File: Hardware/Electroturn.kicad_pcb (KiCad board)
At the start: 2 copper layers, 122 x 83.1 mm, 45 parts, among them Q1 2N2222, U2 RT9193-3.3, U3 74HC4050D

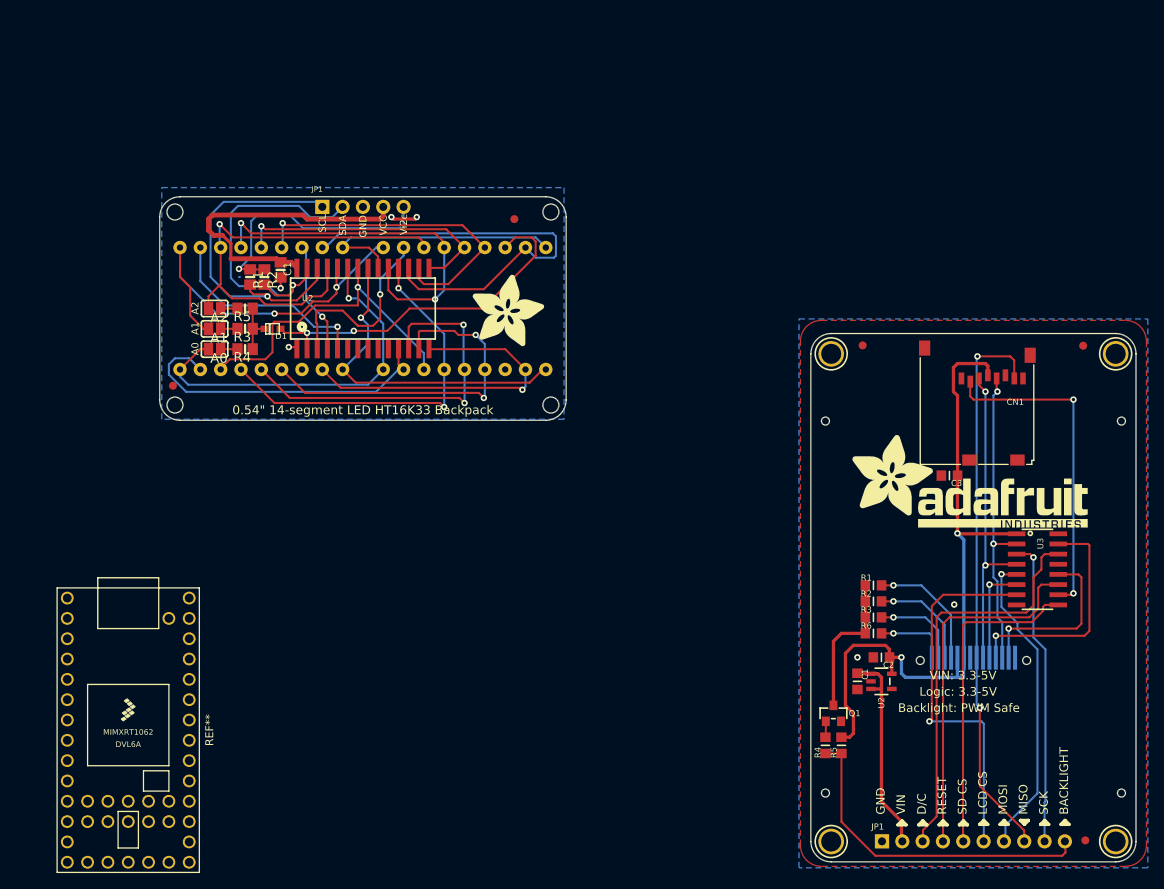
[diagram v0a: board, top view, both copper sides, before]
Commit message: Something like a pcb?
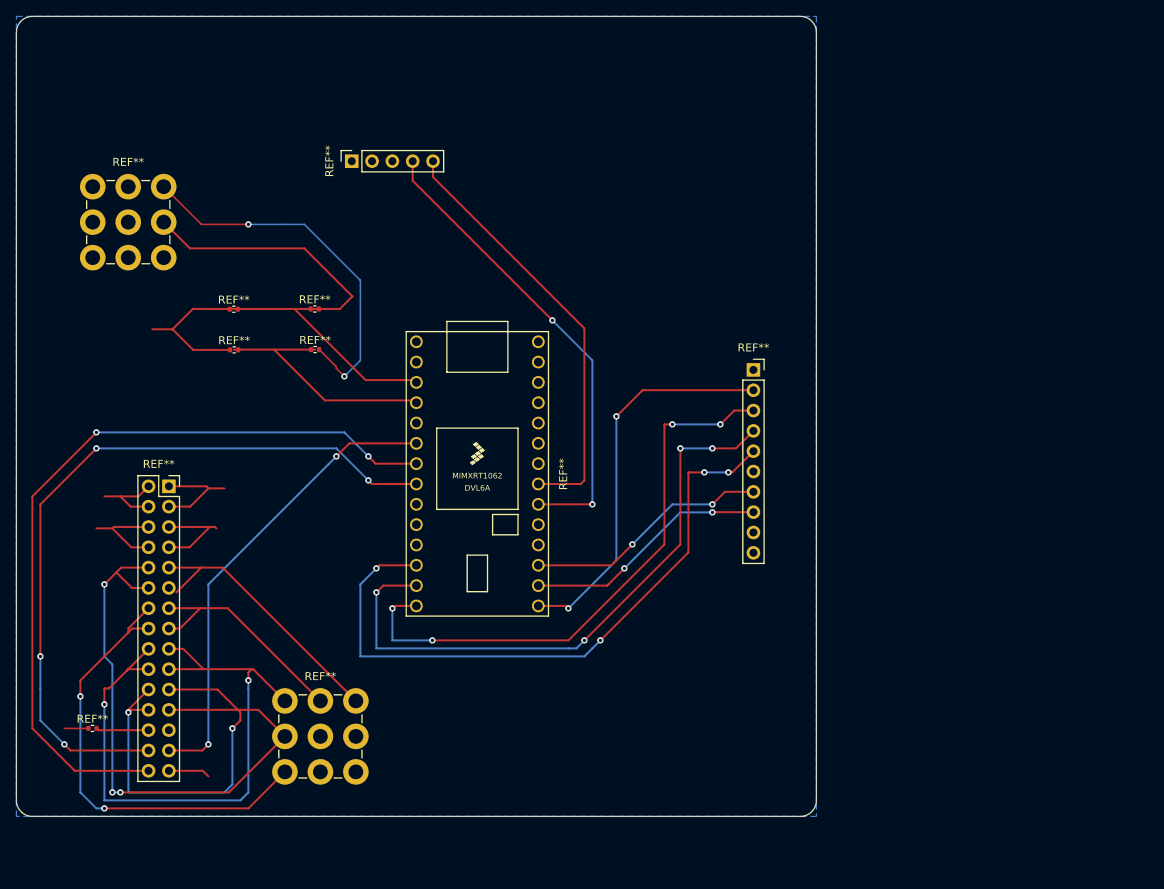
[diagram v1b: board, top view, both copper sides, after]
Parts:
- removed @HOLE0, @HOLE1, @HOLE2, @HOLE3: , 
- removed A0, A1, A2: , Adafruit 0.54 Alphanumeric v0.1:SOLDERJUMPER_REFLOW_NOPASTE
- removed C1: 10uF, Adafruit 0.54 Alphanumeric v0.1:0805-NO
- removed C1, C2, C3: 10uF, Adafruit_2.2_SPI_240x320:_0805MP
- removed CN1: , Adafruit_2.2_SPI_240x320:MICROSD
- removed D1: 1N4148, Adafruit 0.54 Alphanumeric v0.1:SOD-323F
- removed FID1, FID2, FID3: FIDUCIAL"", Adafruit_2.2_SPI_240x320:FIDUCIAL_1MM
- removed JP1: , Adafruit 0.54 Alphanumeric v0.1:1X05_ROUND_70
- removed JP1: , Adafruit_2.2_SPI_240x320:1X10_ROUND70
- removed LED1, LED2: , Adafruit 0.54 Alphanumeric v0.1:SEGMENT_STARTBUST_DUAL_KWA-541CBB
- removed Q1: 2N2222, Adafruit_2.2_SPI_240x320:SOT23-WIDE
- removed R1, R2: 10K, Adafruit 0.54 Alphanumeric v0.1:0805-NO
- removed R1, R2, R3, R6: 10, Adafruit_2.2_SPI_240x320:_0805MP
- removed R3, R4, R5: 47K, Adafruit 0.54 Alphanumeric v0.1:0805-NO
- removed R4: 1K, Adafruit_2.2_SPI_240x320:_0805MP
- removed R5: 10K, Adafruit_2.2_SPI_240x320:_0805MP
- removed U$1, U$2: FIDUCIAL, Adafruit 0.54 Alphanumeric v0.1:FIDUCIAL_1MM
- removed U$2, U$3, U$4, U$5: MOUNTINGHOLE2.5, Adafruit_2.2_SPI_240x320:MOUNTINGHOLE_2.5_PLATED
- removed U$20: , Adafruit_2.2_SPI_240x320:ADAFRUIT_TEXT_30MM
- removed U$3: , Adafruit 0.54 Alphanumeric v0.1:ADAFRUIT_9MM
- removed U1: , Adafruit_2.2_SPI_240x320:TM022HDH26_2.2IN_LCD
- removed U2: , Adafruit 0.54 Alphanumeric v0.1:SOP28_300MIL
- removed U2: RT9193-3.3, Adafruit_2.2_SPI_240x320:SOT23-5
- removed U3: 74HC4050D, Adafruit_2.2_SPI_240x320:SOIC16
- added REF**: Gecko G250x, Connector_PinSocket_2.54mm:PinSocket_2x15_P2.54mm_Vertical, F.Cu at (99.1, 78.7)
- added REF**: Alphanumeric, Connector_PinSocket_2.54mm:PinSocket_1x05_P2.54mm_Vertical, F.Cu at (121.9, 38.1)
- added REF**: Screw Terminal, TerminalBlock_Wuerth:Wuerth_REDCUBE-THR_WP-THRBU_74650194_THR, F.Cu at (118.0, 110.0)
- added REF**: 5k, Resistor_SMD:R_0402_1005Metric, F.Cu at (117.3, 56.6)
- added REF**: Screw Terminal, TerminalBlock_Wuerth:Wuerth_REDCUBE-THR_WP-THRBU_74650194_THR, F.Cu at (94.0, 45.7)
- added REF**: 10k, Resistor_SMD:R_0402_1005Metric, F.Cu at (107.2, 61.7)
- added REF**: 5k, Resistor_SMD:R_0402_1005Metric, F.Cu at (117.3, 61.6)
- added REF**: TFT Display, Connector_PinSocket_2.54mm:PinSocket_1x10_P2.54mm_Vertical, F.Cu at (172.1, 64.2)
- added REF**: 10k, Resistor_SMD:R_0402_1005Metric, F.Cu at (107.2, 56.6)
- added REF**: 2.8k, Resistor_SMD:R_0402_1005Metric, F.Cu at (89.5, 109.0)
- moved REF** 54.1 mm to (137.6, 77.2)
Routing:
- net (no net): track 1691.0 -> 1259.2 mm, vias 51 -> 40
- removed copper zone on F.Cu, net (none)
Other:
- board size 122 x 83.1 mm -> 100 x 100 mm
- board text removed: "+"
- board text removed: "-"
- board text removed: "0.54" 14-segment LED HT16K33 Backpack"
- board text removed: "240x320 2.2" TFT w/ILI9340C"
- board text removed: "A0"
- board text removed: "A1"
- board text removed: "A2"
- board text removed: "BACKLIGHT"
- board text removed: "BL"
- board text removed: "Backlight: PWM Safe"
- board text removed: "C"
- board text removed: "CS"
- board text removed: "D"
- board text removed: "D/C"
- board text removed: "GND"
- board text removed: "LCD CS"
- board text removed: "Logic: 3.3-5V"
- board text removed: "MISO"
- board text removed: "MOSI"
- board text removed: "RESET"
- board text removed: "RST"
- board text removed: "SCK"
- board text removed: "SCL"
- board text removed: "SD CS"
- board text removed: "SDA"
- board text removed: "SDCS"
- board text removed: "VCC"
- board text removed: "VIN"
- board text removed: "VIN: 3.3-5V"
- board text removed: "Vi2c"
- board text removed: "by adafruit!"
